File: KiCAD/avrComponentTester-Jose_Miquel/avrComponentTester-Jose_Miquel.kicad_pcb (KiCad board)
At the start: 2 copper layers, 14 parts, among them Q1 2N3904, Q2 2N3904, Q3 2N3906, U1 ST7735_1.8

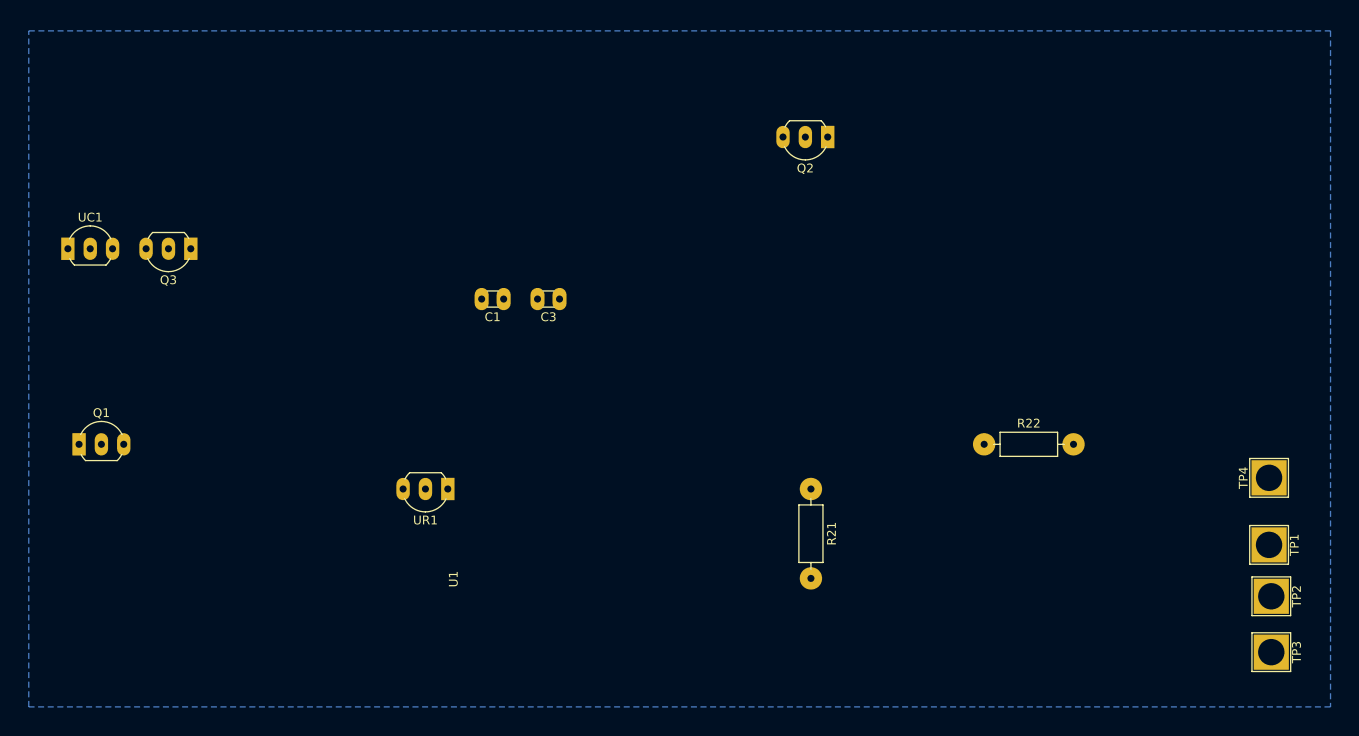
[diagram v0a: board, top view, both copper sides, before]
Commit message: kicad6
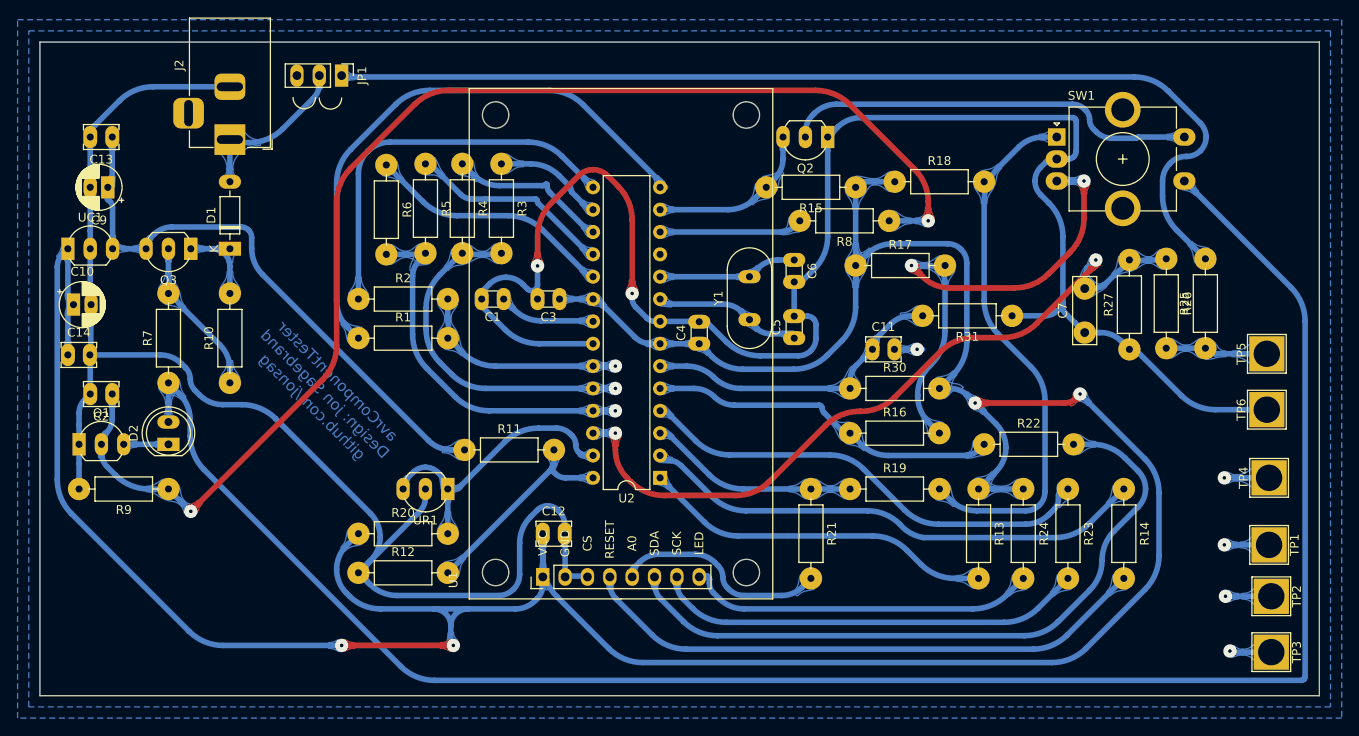
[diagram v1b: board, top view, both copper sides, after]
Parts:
- added C10: 10u, My_Misc:CP_Radial_D5.0mm_P2.00mm_larger, F.Cu at (90.2, 85.7)
- added C11: 100n, My_Misc:C_Disc_D3.8mm_W2.6mm_P2.50mm_large, F.Cu at (181.0, 90.8)
- added C12: 100n, My_Misc:C_Disc_D3.8mm_W2.6mm_P2.50mm_large, F.Cu at (143.5, 111.8)
- added C13: 100n, My_Misc:C_Disc_D3.8mm_W2.6mm_P2.50mm_large, F.Cu at (94.6, 66.7)
- added C14: 100n, My_Misc:C_Disc_D3.8mm_W2.6mm_P2.50mm_large, F.Cu at (89.5, 91.4)
- added C2: 10n, My_Misc:C_Disc_D3.8mm_W2.6mm_P2.50mm_large, F.Cu at (94.6, 95.9)
- added C4: 100n, My_Misc:C_Disc_D3.0mm_W1.6mm_P2.50mm_larg, F.Cu at (161.3, 90.2)
- added C5: 22p, My_Misc:C_Disc_D3.0mm_W1.6mm_P2.50mm_larg, F.Cu at (172.1, 89.5)
- added C6: 22p, My_Misc:C_Disc_D3.0mm_W1.6mm_P2.50mm_larg, F.Cu at (172.1, 80.6)
- added C7: 10n 100V, My_Misc:C_Disc_D7.5mm_W2.5mm_P5.00mm_larger, F.Cu at (205.1, 88.9)
- added C9: 10u, My_Misc:CP_Radial_D5.0mm_P2.00mm_larger, F.Cu at (94.1, 72.4)
- added D1: D_Schottky, My_Misc:D_DO-35_SOD27_P7.62mm_Horizontal_large, F.Cu at (108.0, 79.4)
- added D2: LED, My_Misc:LED_D5.0mm_larger_pads, F.Cu at (101.0, 101.6)
- added J2: 8-15VDC In, Connector_BarrelJack:BarrelJack_Horizontal, F.Cu at (108.0, 67.0)
- added JP1: Vext <50V, Zener < VCC, My_Parts:Jumper_1x03_P2.54mm_large, F.Cu at (120.7, 59.7)
- added R1: 680R, My_Misc:R_Axial_DIN0207_L6.3mm_D2.5mm_P10.16mm_Horizontal_larger_pads, F.Cu at (122.6, 89.5)
- added R10: 33k, My_Misc:R_Axial_DIN0207_L6.3mm_D2.5mm_P10.16mm_Horizontal_larger_pads, F.Cu at (108.0, 94.6)
- added R11: 10k, My_Misc:R_Axial_DIN0207_L6.3mm_D2.5mm_P10.16mm_Horizontal_larger_pads, F.Cu at (134.6, 102.2)
- added R12: 3k3, My_Misc:R_Axial_DIN0207_L6.3mm_D2.5mm_P10.16mm_Horizontal_larger_pads, F.Cu at (122.6, 116.2)
- added R13: 10k, My_Misc:R_Axial_DIN0207_L6.3mm_D2.5mm_P10.16mm_Horizontal_larger_pads, F.Cu at (193.0, 106.7)
- added R14: 10k, My_Misc:R_Axial_DIN0207_L6.3mm_D2.5mm_P10.16mm_Horizontal_larger_pads, F.Cu at (209.6, 106.7)
- added R15: 27k, My_Misc:R_Axial_DIN0207_L6.3mm_D2.5mm_P10.16mm_Horizontal_larger_pads, F.Cu at (179.1, 72.4)
- added R16: 1k, My_Misc:R_Axial_DIN0207_L6.3mm_D2.5mm_P10.16mm_Horizontal_larger_pads, F.Cu at (178.4, 100.3)
- added R17: 10k, My_Misc:R_Axial_DIN0207_L6.3mm_D2.5mm_P10.16mm_Horizontal_larger_pads, F.Cu at (179.1, 81.3)
- added R18: 10k, My_Misc:R_Axial_DIN0207_L6.3mm_D2.5mm_P10.16mm_Horizontal_larger_pads, F.Cu at (183.5, 71.8)
- added R19: 1k, My_Misc:R_Axial_DIN0207_L6.3mm_D2.5mm_P10.16mm_Horizontal_larger_pads, F.Cu at (178.4, 106.7)
- added R2: 470k, My_Misc:R_Axial_DIN0207_L6.3mm_D2.5mm_P10.16mm_Horizontal_larger_pads, F.Cu at (122.6, 85.1)
- added R20: 2k2, My_Misc:R_Axial_DIN0207_L6.3mm_D2.5mm_P10.16mm_Horizontal_larger_pads, F.Cu at (122.6, 111.8)
- added R23: 10k, My_Misc:R_Axial_DIN0207_L6.3mm_D2.5mm_P10.16mm_Horizontal_larger_pads, F.Cu at (203.2, 106.7)
- added R24: 220R, My_Misc:R_Axial_DIN0207_L6.3mm_D2.5mm_P10.16mm_Horizontal_larger_pads, F.Cu at (198.1, 106.7)
- added R25: 2k2, My_Misc:R_Axial_DIN0207_L6.3mm_D2.5mm_P10.16mm_Horizontal_larger_pads, F.Cu at (218.8, 90.7)
- added R26: 179k45, My_Misc:R_Axial_DIN0207_L6.3mm_D2.5mm_P10.16mm_Horizontal_larger_pads, F.Cu at (214.4, 80.5)
- added R27: 20k, My_Misc:R_Axial_DIN0207_L6.3mm_D2.5mm_P10.16mm_Horizontal_larger_pads, F.Cu at (210.2, 90.8)
- added R3: 680R, My_Misc:R_Axial_DIN0207_L6.3mm_D2.5mm_P10.16mm_Horizontal_larger_pads, F.Cu at (138.8, 69.7)
- added R30: 10k, My_Misc:R_Axial_DIN0207_L6.3mm_D2.5mm_P10.16mm_Horizontal_larger_pads, F.Cu at (178.4, 95.2)
- added R31: 10k, My_Misc:R_Axial_DIN0207_L6.3mm_D2.5mm_P10.16mm_Horizontal_larger_pads, F.Cu at (196.8, 87.0)
- added R4: 470k, My_Misc:R_Axial_DIN0207_L6.3mm_D2.5mm_P10.16mm_Horizontal_larger_pads, F.Cu at (134.4, 69.7)
- added R5: 680R, My_Misc:R_Axial_DIN0207_L6.3mm_D2.5mm_P10.16mm_Horizontal_larger_pads, F.Cu at (130.2, 69.7)
- added R6: 470k, My_Misc:R_Axial_DIN0207_L6.3mm_D2.5mm_P10.16mm_Horizontal_larger_pads, F.Cu at (125.7, 69.8)
- added R7: 3k3, My_Misc:R_Axial_DIN0207_L6.3mm_D2.5mm_P10.16mm_Horizontal_larger_pads, F.Cu at (101.0, 94.6)
- added R8: 27k, My_Misc:R_Axial_DIN0207_L6.3mm_D2.5mm_P10.16mm_Horizontal_larger_pads, F.Cu at (182.9, 76.2)
- added R9: 100k, My_Misc:R_Axial_DIN0207_L6.3mm_D2.5mm_P10.16mm_Horizontal_larger_pads, F.Cu at (101.0, 106.7)
- added SW1: EC11, My_Misc:RotaryEncoder_Alps_EC11E-Switch_Vertical_H20mm_CircularMountingHoles_large, F.Cu at (201.9, 66.7)
- added TP5: TestPoint, My_Parts:TestPoint_THTPad_4.0x4.0mm_Drill3.0mm, F.Cu at (225.8, 91.3)
- added TP6: TestPoint, My_Parts:TestPoint_THTPad_4.0x4.0mm_Drill3.0mm, F.Cu at (225.8, 97.7)
- added U2: ATmega328P-PU, Package_DIP:DIP-28_W7.62mm, F.Cu at (156.8, 105.4)
- added Y1: 8MHz, My_Misc:Crystal_HC49-4H_Vertical_large, F.Cu at (167.0, 87.4)
- U1: value ST7735_1.8 -> ST7735_1.8"_TFT_128x160_w_SD-card; footprint My_Parts:ST7735_1.8_TFT_display_128x160_no-SD_large -> My_Parts:ST7735_1.8_TFT_display_128x160_w_SD-card_no_SD_pins_large
- moved U1 0.10 mm to (143.5, 116.7)
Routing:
- net +5V: track 0.00 -> 368.0 mm, vias 0 -> 4
- net TPGND: track 0.00 -> 356.3 mm, vias 0 -> 2
- net Net-(D2-Pad2): track 0.00 -> 210.4 mm
- net Net-(C2-Pad1): track 0.00 -> 147.6 mm, vias 0 -> 2
- net Net-(JP1-Pad1): track 0.00 -> 119.8 mm
- net ZenerMeas: track 0.00 -> 85.6 mm, vias 0 -> 2
- net Net-(R22-Pad2): track 0.00 -> 79.0 mm
- net Net-(R14-Pad2): track 0.00 -> 65.6 mm
- net VREF: track 0.00 -> 65.5 mm
- net Net-(R1-Pad1): track 0.00 -> 65.3 mm
- net Net-(R18-Pad2): track 0.00 -> 61.5 mm
- net RST: track 0.00 -> 57.6 mm
- net Net-(R16-Pad2): track 0.00 -> 55.5 mm, vias 0 -> 2
- net SCK: track 0.00 -> 53.0 mm
- net Net-(R23-Pad2): track 0.00 -> 49.2 mm
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- added copper zone on B.Cu, net (none)
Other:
- board outline added: 145.4 x 74.3 mm
- net class Default removed
- board text added: "avrComponentTester Design: jon Sagebrand github.com/jonsag"
